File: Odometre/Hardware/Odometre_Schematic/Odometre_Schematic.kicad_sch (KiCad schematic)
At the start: 29 parts, among them IC1 STM32C092FCP6, J1 Conn_01x03_Pin, J2 Conn_01x03_Pin, J3 Conn_Alim, J4 Conn_Laser1, J5 Conn_Laser2, J6 Conn_01x06_Pin, J7 Conn_01x06_Pin, SW1 Reset_Botton, SW2 Debug_Botton, U1 MCP2562-E-SN, U2 LM1117DT-3.3

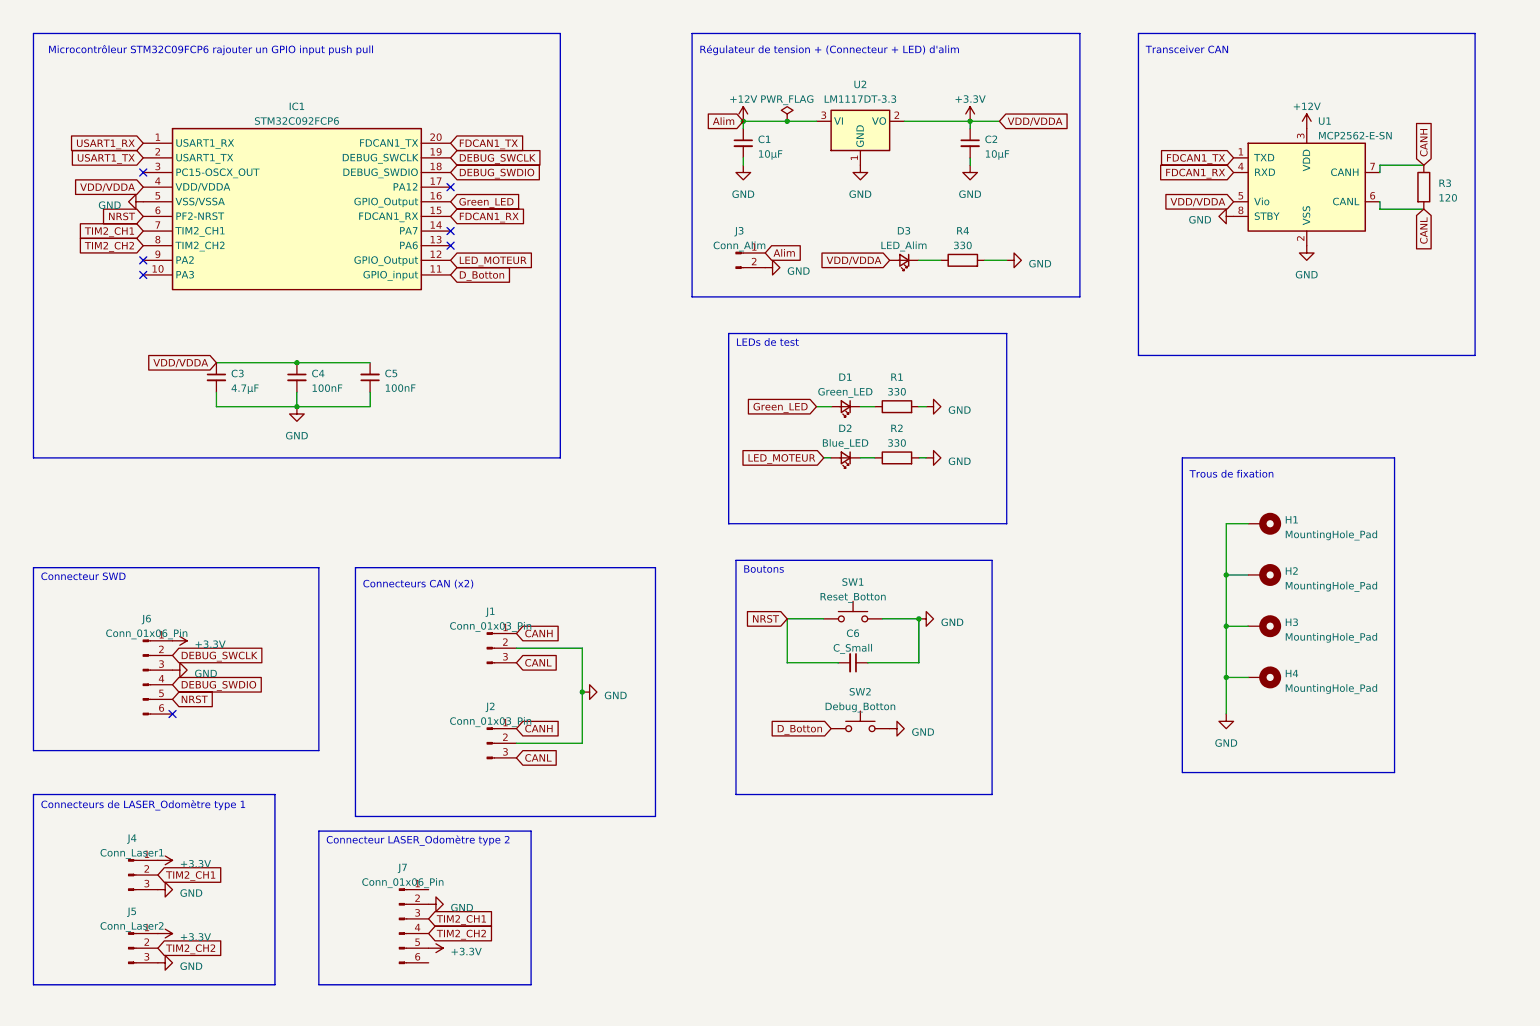
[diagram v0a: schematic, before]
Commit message: modif shematic
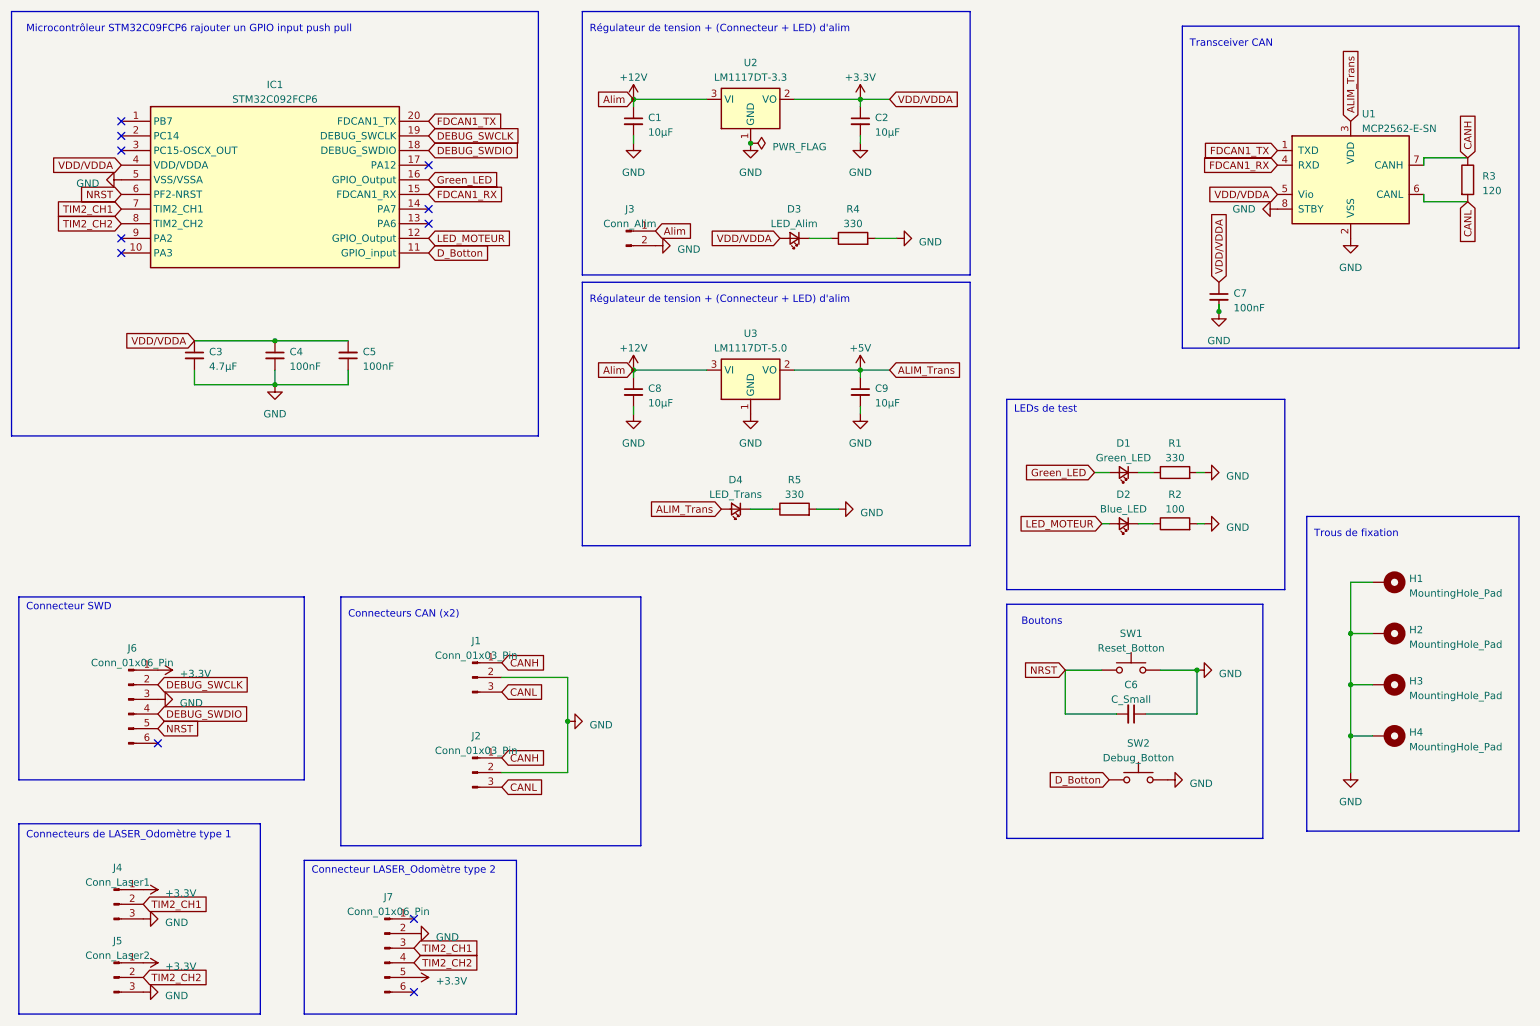
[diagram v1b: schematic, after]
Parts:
- added C7: 100nF, symbol Device:C_Small
- added C8, C9: 10µF, Capacitor_SMD:C_0805_2012Metric_Pad1.18x1.45mm_HandSolder, symbol Device:C_Small
- added D4: LED_Trans, symbol Device:LED_Small
- added R5: 330, symbol Device:R
- added U3: LM1117DT-5.0, Package_TO_SOT_SMD:TO-252-3_TabPin2, symbol Regulator_Linear:LM1117DT-5.0
- R2: value 330 -> 100
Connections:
- net +12V: now also C8.1, C9.1, D4.2 (A), U3.2 (VO), U3.3 (VI)
- net +3.3V: now also C7.1
- net GND: now also C7.2, C8.2, C9.2, R5.2, U3.1 (GND)
- net USART1_RX: no longer names the net of IC1.1 (PB7)
- net USART1_TX: no longer names the net of IC1.2 (PC14)
- new net: D4.1 (K), R5.1
- no-connect marks 7 -> 11
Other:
- moved on the sheet: C1, C2, C3, C4, C5, C6, D1, D2, D3, H1, H2, H3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
